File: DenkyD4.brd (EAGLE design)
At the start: 33.2 x 25.7 mm, 43 parts, among them J1 CON_HEADER_1X06NO_SILK, J2 CON_HEADER_1X06NO_SILK, Q1 MUN5214DW1T1G, Q2 BSS138, SW1 RESET, U1 ESP32-PICO-D4, U2 FT231XQ-R, U3 AP2112K

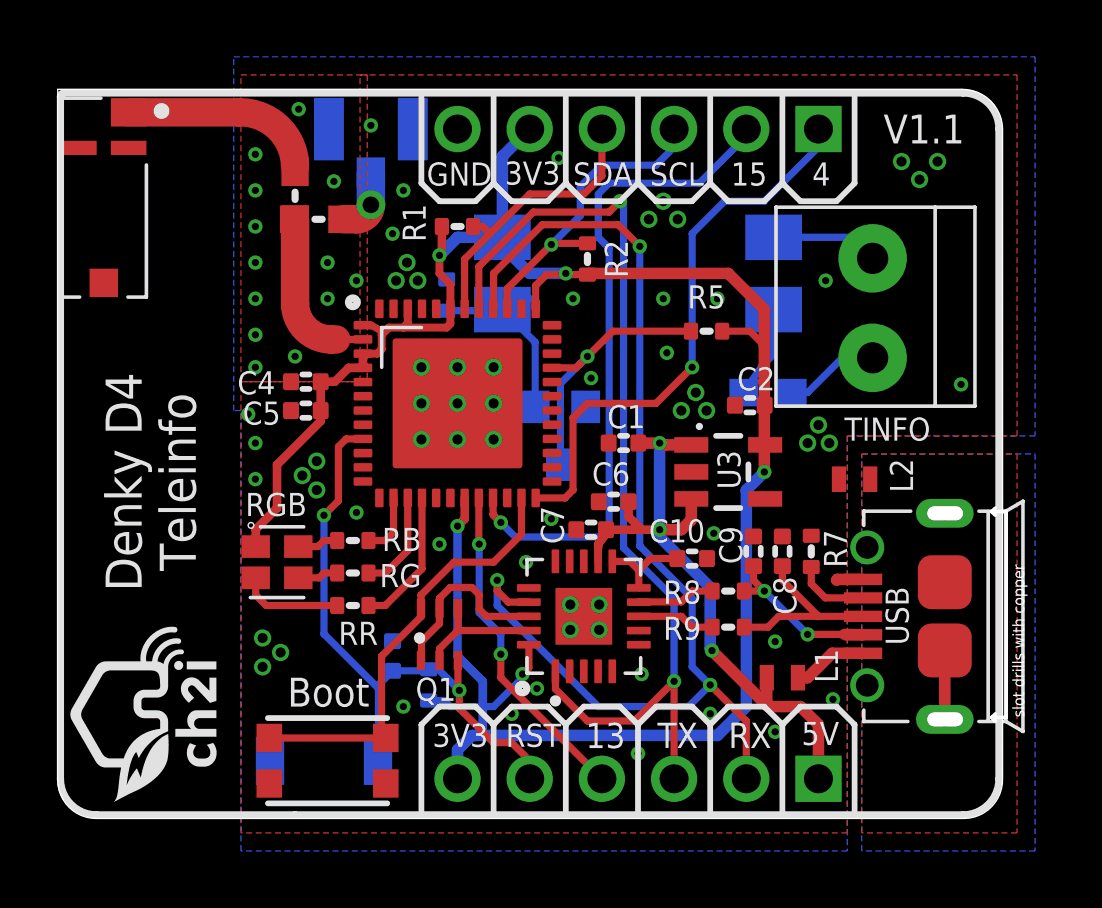
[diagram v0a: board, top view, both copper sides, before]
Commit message: Updated to V1.2
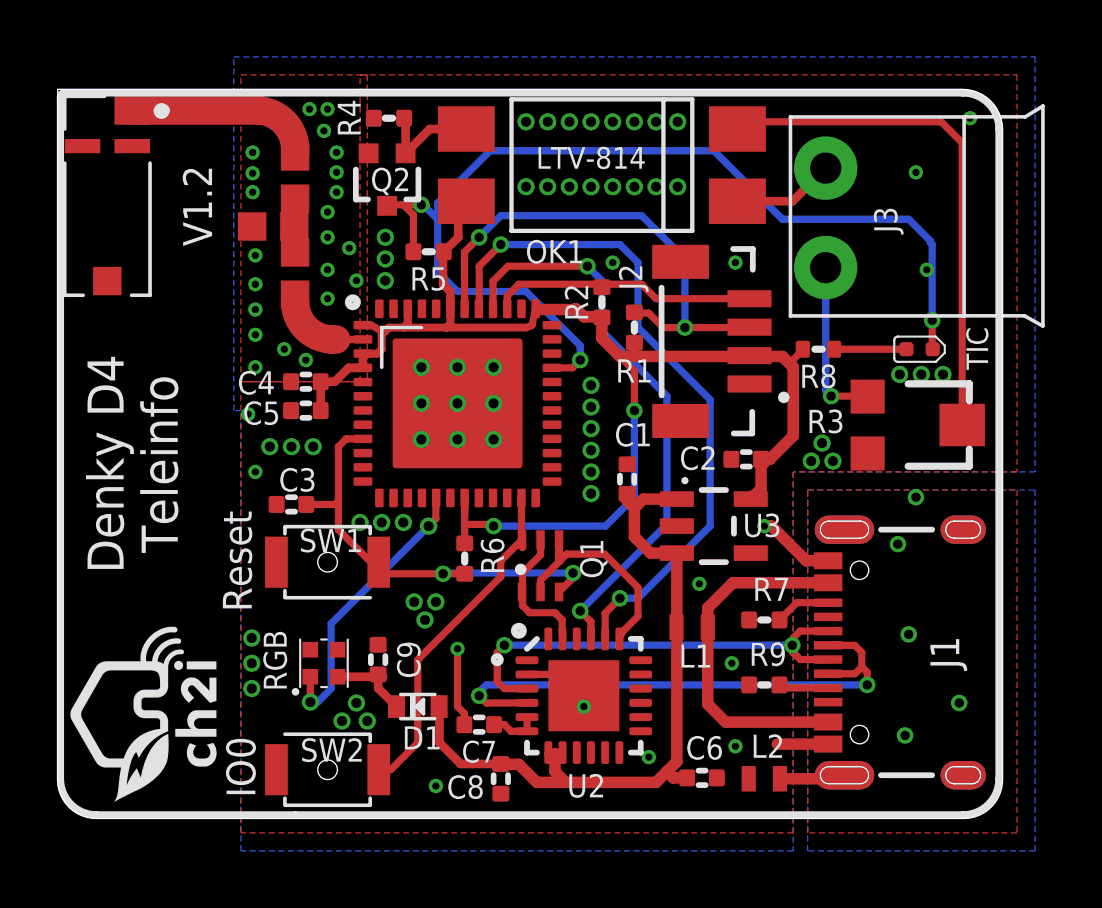
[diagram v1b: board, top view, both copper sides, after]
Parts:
- removed C10: 100nF, _c2h:0402-CAP-OK
- removed E1: NN03-320, _c2h:XCVR_NN03-320
- removed R10, R11: 0R, _c2h:0603-RES
- removed RB, RG: 150, _c2h:0402-RES
- removed RGB: ASMB-KTF0-0A306, Particle:PLCC4-2MM-RGB
- removed RR: 330, _c2h:0402-RES
- removed TINFO: 1X2-3.5MM, adafruit:1X2-3.5MM
- removed UFL: U.FL-R-SMT-1, Kris:U.FL-R-SMT-1
- removed USB: ZX62-B-5PA, Seeed-Connector:MICRO-USB5+6P-SMD-0.65-AB
- added ANT: NN01-102, _c2h:XCVR_NN03-320
- added D1: 1N4148, microbuilder:SOD-523
- added J3: KF2EDGR-3.81-2P, _c2h:1X2-3.5MM
- added LED: SK68051515, _c2h:SK6805-1515
- added LTIC: BLUE, OPL_Optoelectronics:LED-0402
- added Z1, Z3: 0R, _c2h:0603-MATCHNET
- added Z2: DNP, _c2h:0603-MATCHNET
- C3, C5: value 0.1uF -> 100nF
- C8, C9: value 47pF -> 100nF
- J1: value CON_HEADER_1X06NO_SILK -> US Type C; device _c2h:M1X6_NO_SILK -> SparkFun-Connectors:USB-C-16P-4LAYER-ISOLATED
- J2: value CON_HEADER_1X06NO_SILK -> Vertical Qwiic Connector; device _c2h:M1X6_NO_SILK -> _c2h:JST04_1MM_VERT
- Q2: device Seeed-Discrete:SOT23 -> _c2h:SOT-323-3
- R3: value 220 -> 1K; device _c2h:0603-RES -> adafruit:TC33X
- R5: value 10k -> 10K
- R7: value 100K -> 5.1K
- R8: value 27 -> 470; device _c2h:0402-RES -> LowPowerLab:0402-RES
- R9: value 27 -> 5.1K
- SW1: device Seeed-Switch:SW2-2.6-3.0X2.5X1.2+0.4MM -> _c2h:C498294
- SW2: device microbuilder:BTN_KMR2_4.6X2.8 -> _c2h:C498294
- U2: value FT231XQ-R -> CH9106; device FT231XQ-R:QFN50P400X400X80-21N -> microbuilder:QFN24_4MM_SMSC
- moved J1 18.8 mm to (40.0, 14.0), turned to 90 degrees
- moved J2 15.5 mm to (34.5, 24.9), turned to 90 degrees
- moved C9 13.7 mm to (20.7, 13.7)
- moved C8 12.7 mm to (25.0, 9.53), turned to 270 degrees
- moved L2 11.0 mm to (34.3, 9.53)
- moved Q2 10.9 mm to (21.0, 30.6), flipped to the top
- moved C6 10.2 mm to (32.1, 9.56), turned to 180 degrees
- moved R5 10.2 mm to (22.5, 28.1)
- moved R8 9.08 mm to (36.2, 24.6), turned to 180 degrees
- moved C7 7.91 mm to (24.3, 11.4)
- moved R1 7.17 mm to (29.7, 25.4), turned to 270 degrees
- moved SW1 6.99 mm to (18.9, 17.1), flipped to the top, turned to 0 degrees
- moved R4 6.55 mm to (21.1, 32.8), flipped to the top, turned to 0 degrees
- moved C3 6.41 mm to (17.7, 19.2), flipped to the top, turned to 180 degrees
- moved R3 5.46 mm to (39.8, 22.0), flipped to the top, turned to 270 degrees
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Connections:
- removed net ANT: R11.2, UFL.P$3
- removed net B$7: RB.2, RGB.BLUE
- removed net DM: C9.1, R8.2, USB.2
- removed net DP: C8.1, R9.2, USB.3
- removed net G$6: RG.2, RGB.GREEN
- removed net GROUND: E1.2
- removed net ID: R7.2, USB.4
- removed net R$2: RGB.RED, RR.2
- removed net VBUS: L1.1, USB.1
- new net 5V: J1.VBUS1, J1.VBUS2, L1.1
- new net N$10: LTIC.+, R8.1
- new net N$11: J1.A5, R9.2
- new net N$12: J1.B5, R7.2
- new net N$6: U2.1
- new net N$8: C7.2, U2.5, U2.6
- new net VLED: C9.1, D1.K, LED.2
- net 3V3: now also J2.2, R8.2; no longer J1.5, J2.6, RGB.CA, U2.20
- net D+: now also J1.A6, J1.B6, U2.3; no longer R8.1, U2.9
- net D-: now also J1.A7, J1.B7, U2.4; no longer R9.1, U2.8
- net DTR: now also U2.23; no longer U2.18
- net GND: now also J1.GND, J1.GND2, J2.1, LED.4, R9.1, SW2.2, U2.2, U2.THERM, Z2.2; no longer C10.2, J1.6, SW2.A, SW2.A', U2.13, U2.21, U2.3, UFL.P$1, UFL.P$2, USB.5
- net GPIO0: now also SW2.1; no longer SW2.B, SW2.B'
- net GPIO13: no longer J2.4
- net GPIO14: now also LED.1
- net GPIO15: no longer J1.2
- net GPIO25: no longer RB.1
- net GPIO26: no longer RG.1
- net GPIO27: no longer RR.1
- net GPIO4: no longer J1.1
- net GPIO8: now also LTIC.-
- net LNA_IN: now also Z3.2; no longer R10.1, R11.1
- net N$1: now also Z1.1, Z2.1, Z3.1; no longer C10.1, U2.10, U2.11
- net N$13: now also ANT.3, Z1.2; no longer E1.3, R10.2
- net N$3: now also R3.2; no longer R3.1
- net N$4: now also J3.1; no longer TINFO.1
- net N$5: now also J3.2, R3.1; no longer R3.2, TINFO.2
- net RESET: no longer J2.5
- net RXD: now also U2.21; no longer J2.2, U2.17
- net SCL: now also J2.4; no longer J1.3
- net SDA: now also J2.3; no longer J1.4
- net SHIELD: now also J1.SHLD1, J1.SHLD2, J1.SHLD3, J1.SHLD4, J1.SHLD5, J1.SHLD6, J1.SHLD7, J1.SHLD8; no longer USB.P1, USB.P2, USB.P3, USB.P4, USB.P5, USB.P6
- net TXD: now also U2.20; no longer J2.3, U2.1
- net V_USB: now also C8.1, D1.A, U2.7, U2.8; no longer C7.2, J2.1, U2.12
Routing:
- net 3V3: track 79.3 -> 47.9 mm, vias 5 -> 2
- net GPIO8: track 9.62 -> 37.2 mm, vias 1 -> 3
- net GPIO15: track 23.7 -> 0.00 mm, vias 1 -> 0
- net GPIO4: track 19.9 -> 0.00 mm, vias 1 -> 0
- net RXD: track 39.5 -> 20.2 mm, vias 3 -> 2
- net D-: track 2.75 -> 19.5 mm, vias 0 -> 2
- net N$3: track 3.29 -> 18.2 mm
- net D+: track 2.76 -> 16.1 mm, vias 0 -> 2
- net 5V: track 0.00 -> 12.5 mm
- net GPIO13: track 11.7 -> 0.00 mm, vias 2 -> 0
- net TXD: track 34.4 -> 23.9 mm
- net GPIO14: track 0.00 -> 10.1 mm, vias 0 -> 2
- net GND: track 0.95 -> 9.91 mm, vias 75 -> 92
- net SDA: track 10.1 -> 17.6 mm, vias 0 -> 2
- net DP: track 6.64 -> 0.00 mm
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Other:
- board text added: "IO0"
- board text added: "TIC"
- board text added: "V1.2"
- board text removed: "13"
- board text removed: "15"
- board text removed: "3V3"
- board text removed: "4"
- board text removed: "5V"
- board text removed: "Boot"
- board text removed: "GND"
- board text removed: "RST"
- board text removed: "RX"
- board text removed: "SCL"
- board text removed: "SDA"
- board text removed: "TX"
- board text removed: "V1.1"
